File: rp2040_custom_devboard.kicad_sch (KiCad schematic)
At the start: 34 parts, among them J1 USB_B_Micro, J2 Conn_02x18_Odd_Even, J3 Conn_02x18_Odd_Even, J4 Conn_01x02, U1 NCP1117-3.3_SOT223, U2 W25Q128JVS, U3 RP2040, Y1 ABM8-272-T3

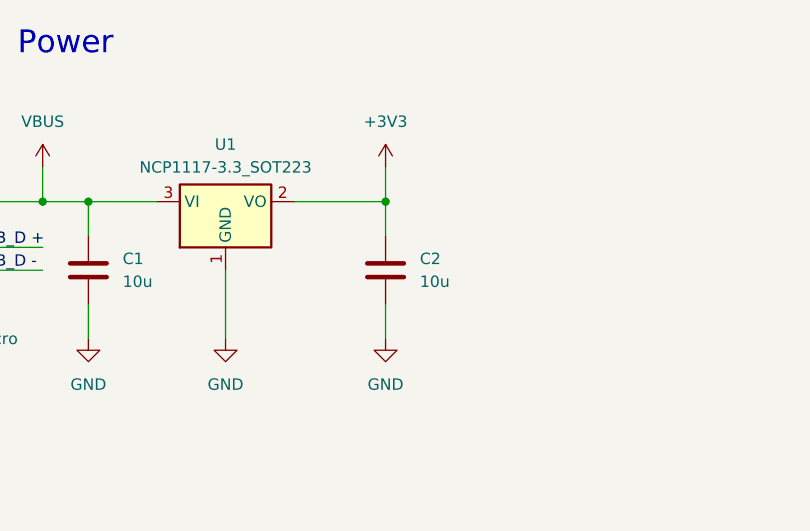
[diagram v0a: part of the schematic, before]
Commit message: REV1
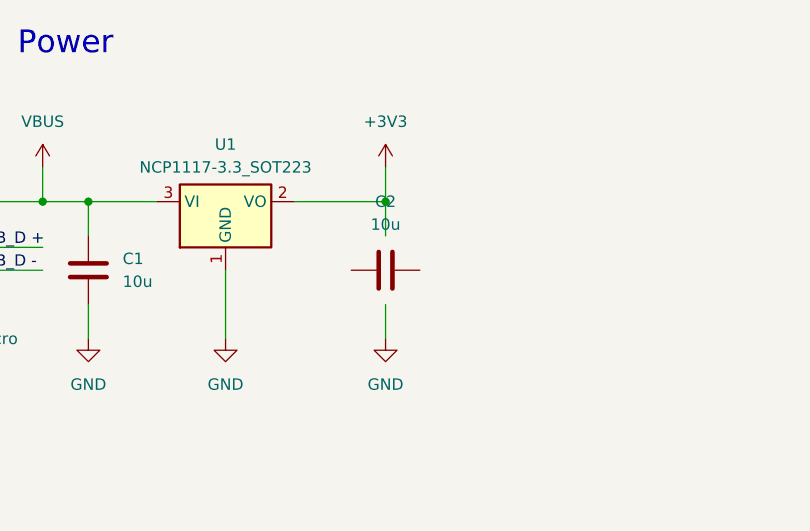
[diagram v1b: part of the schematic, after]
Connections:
- net +3V3: no longer C2.1
- net GND: no longer C2.2
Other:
- moved on the sheet: C2
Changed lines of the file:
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@@
 	(symbol
 		(lib_id "Device:C")
-		(at 88.9 55.88 0)
+		(at 88.9 55.88 90)
 		(unit 1)
 		(exclude_from_sim no)
@@
 		(fields_autoplaced yes)
 		(property "Reference" "C2"
-			(at 92.71 54.6099 0)
+			(at 88.9 48.26 90)
 			(effects
 				(font
 					(size 1.27 1.27)
 				)
-				(justify left)
 			)
 		)
 		(property "Value" "10u"
-			(at 92.71 57.1499 0)
+			(at 88.9 50.8 90)
 			(effects
 				(font
 					(size 1.27 1.27)
 				)
-				(justify left)
 			)
 		)
 		(property "Footprint" "Capacitor_SMD:C_0805_2012Metric"
-			(at 89.8652 59.69 0)
+			(at 92.71 54.9148 0)
 			(effects
 				(font
